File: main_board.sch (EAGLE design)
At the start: 8 parts, among them U1 MAX9019EKA+T

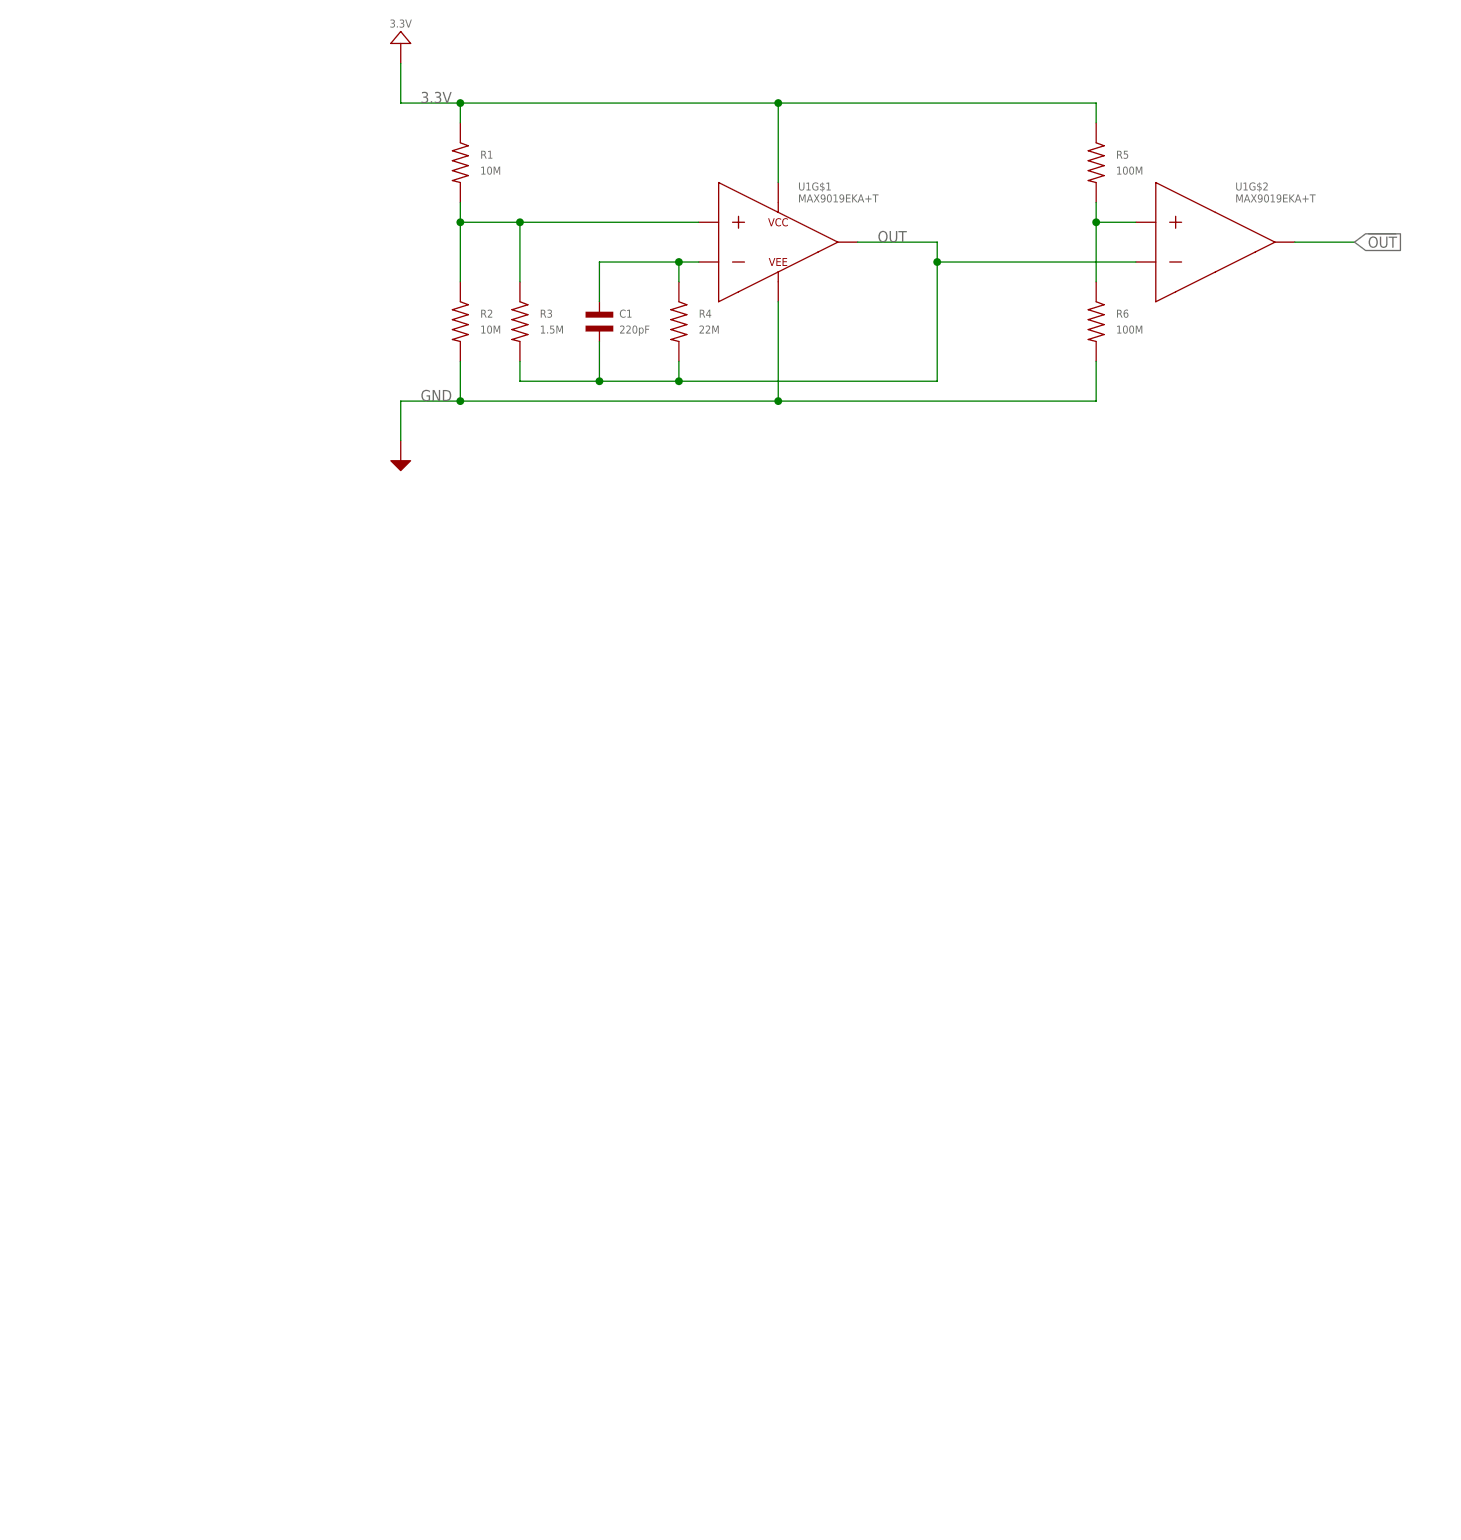
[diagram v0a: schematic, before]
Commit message: working on the solar circuit
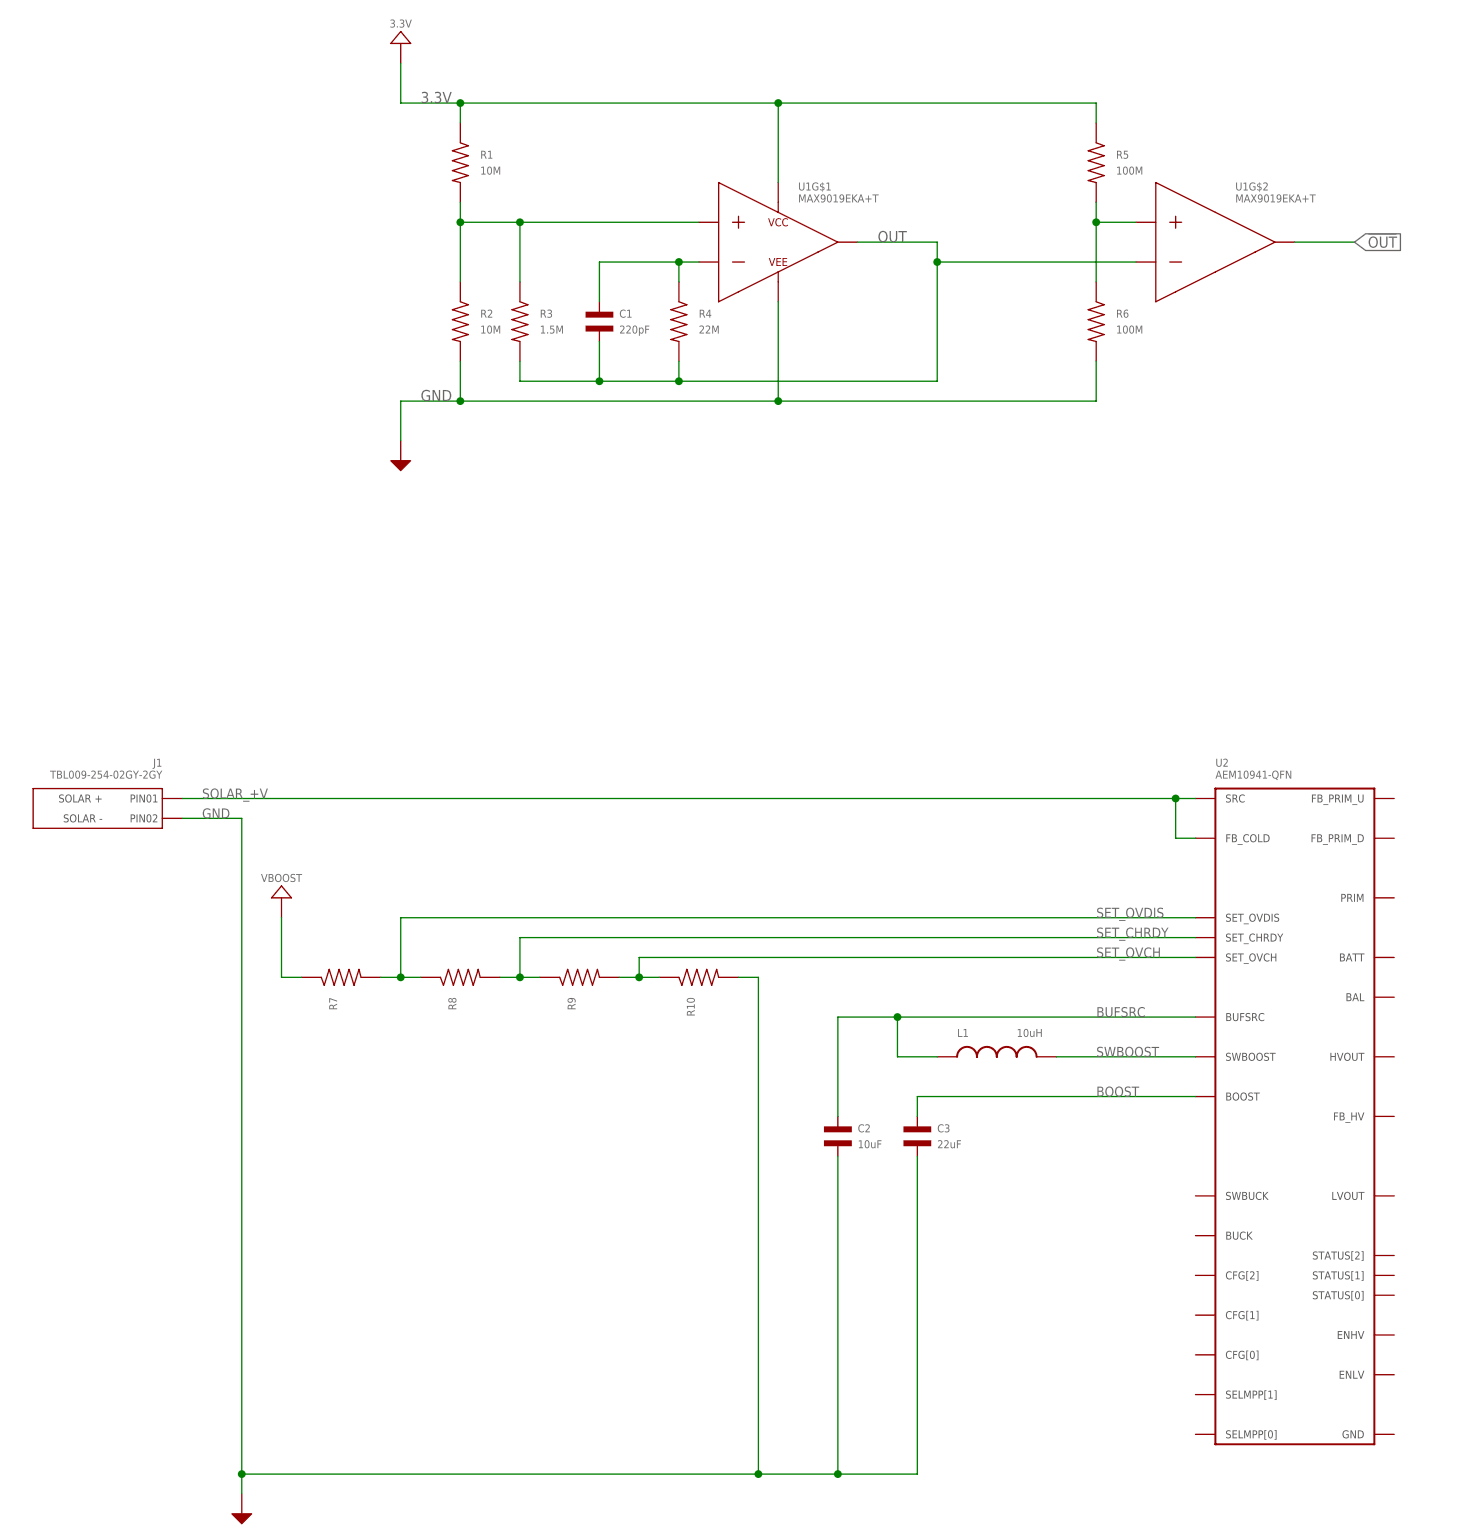
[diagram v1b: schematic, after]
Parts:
- added C2: 10uF, MF_Passives:CAPACITOR_NP_0603
- added C3: 22uF, MF_Passives:CAPACITOR_NP_0603
- added J1: TBL009-254-02GY-2GY, PP_Connectors:CON_01X02_TBL009-254-02GY-2GY
- added L1: 10uH, PP_Passives:INDUCTORLPS4012
- added R10, R7, R8, R9: (no value), MF_Passives:RESISTOR_0805
- added U2: AEM10941-QFN, PP_PowerIC:AEM10941
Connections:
- new net BOOST: C3.P$1, U2.BOOST
- new net BUFSRC: C2.P$1, L1.P$2, U2.BUFSRC
- new net SET_CHRDY: R8.P$2, R9.P$1, U2.SET_CHRDY
- new net SET_OVCH: R10.P$1, R9.P$2, U2.SET_OVCH
- new net SET_OVDIS: R7.P$2, R8.P$1, U2.SET_OVDIS
- new net SOLAR_+V: J1.PIN1, U2.FB_COLD, U2.SRC
- new net SWBOOST: L1.P$1, U2.SWBOOST
- new net VBOOST: R7.P$1
- net GND: now also C2.P$2, C3.P$2, J1.PIN2, R10.P$2
